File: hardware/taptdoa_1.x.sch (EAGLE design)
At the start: 67 parts, among them J1 105017-0001, U1 AP2112K-3.3TRG1, U2 STM32F103RBT6, Y1 8MHz

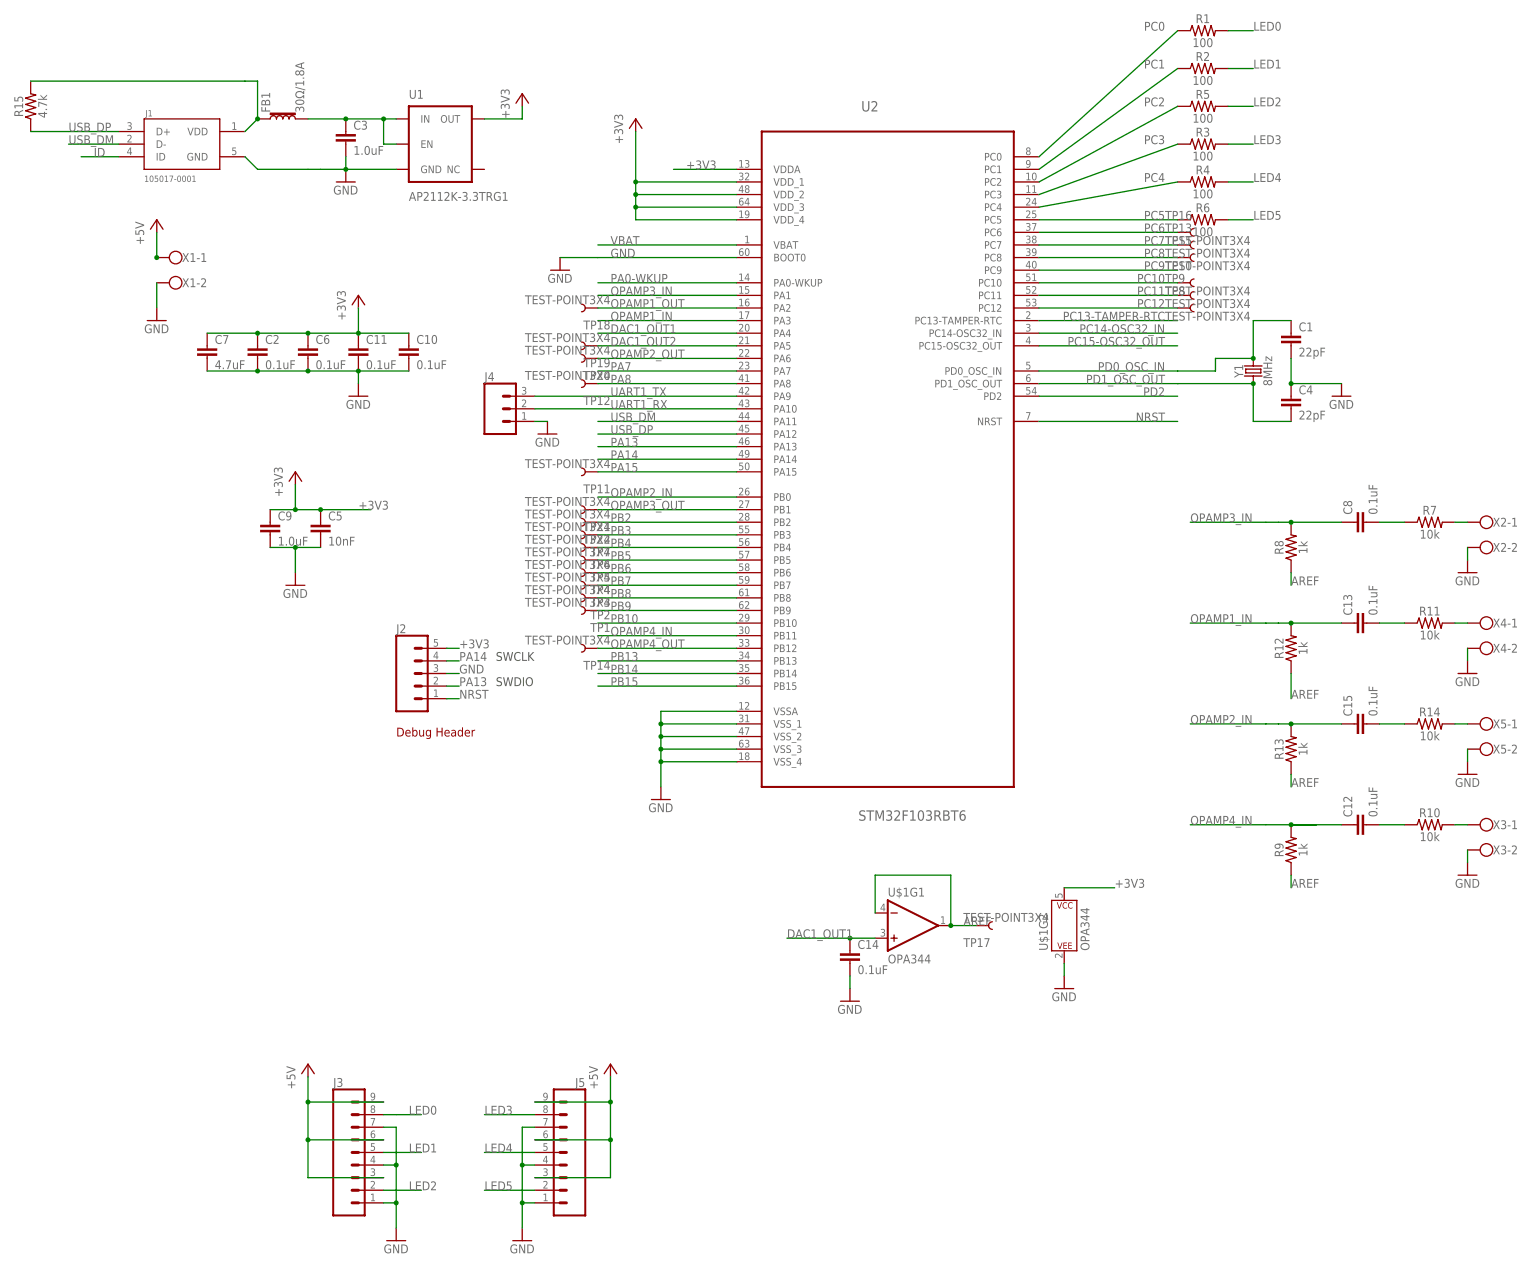
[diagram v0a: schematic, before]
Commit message: v1.2 of board
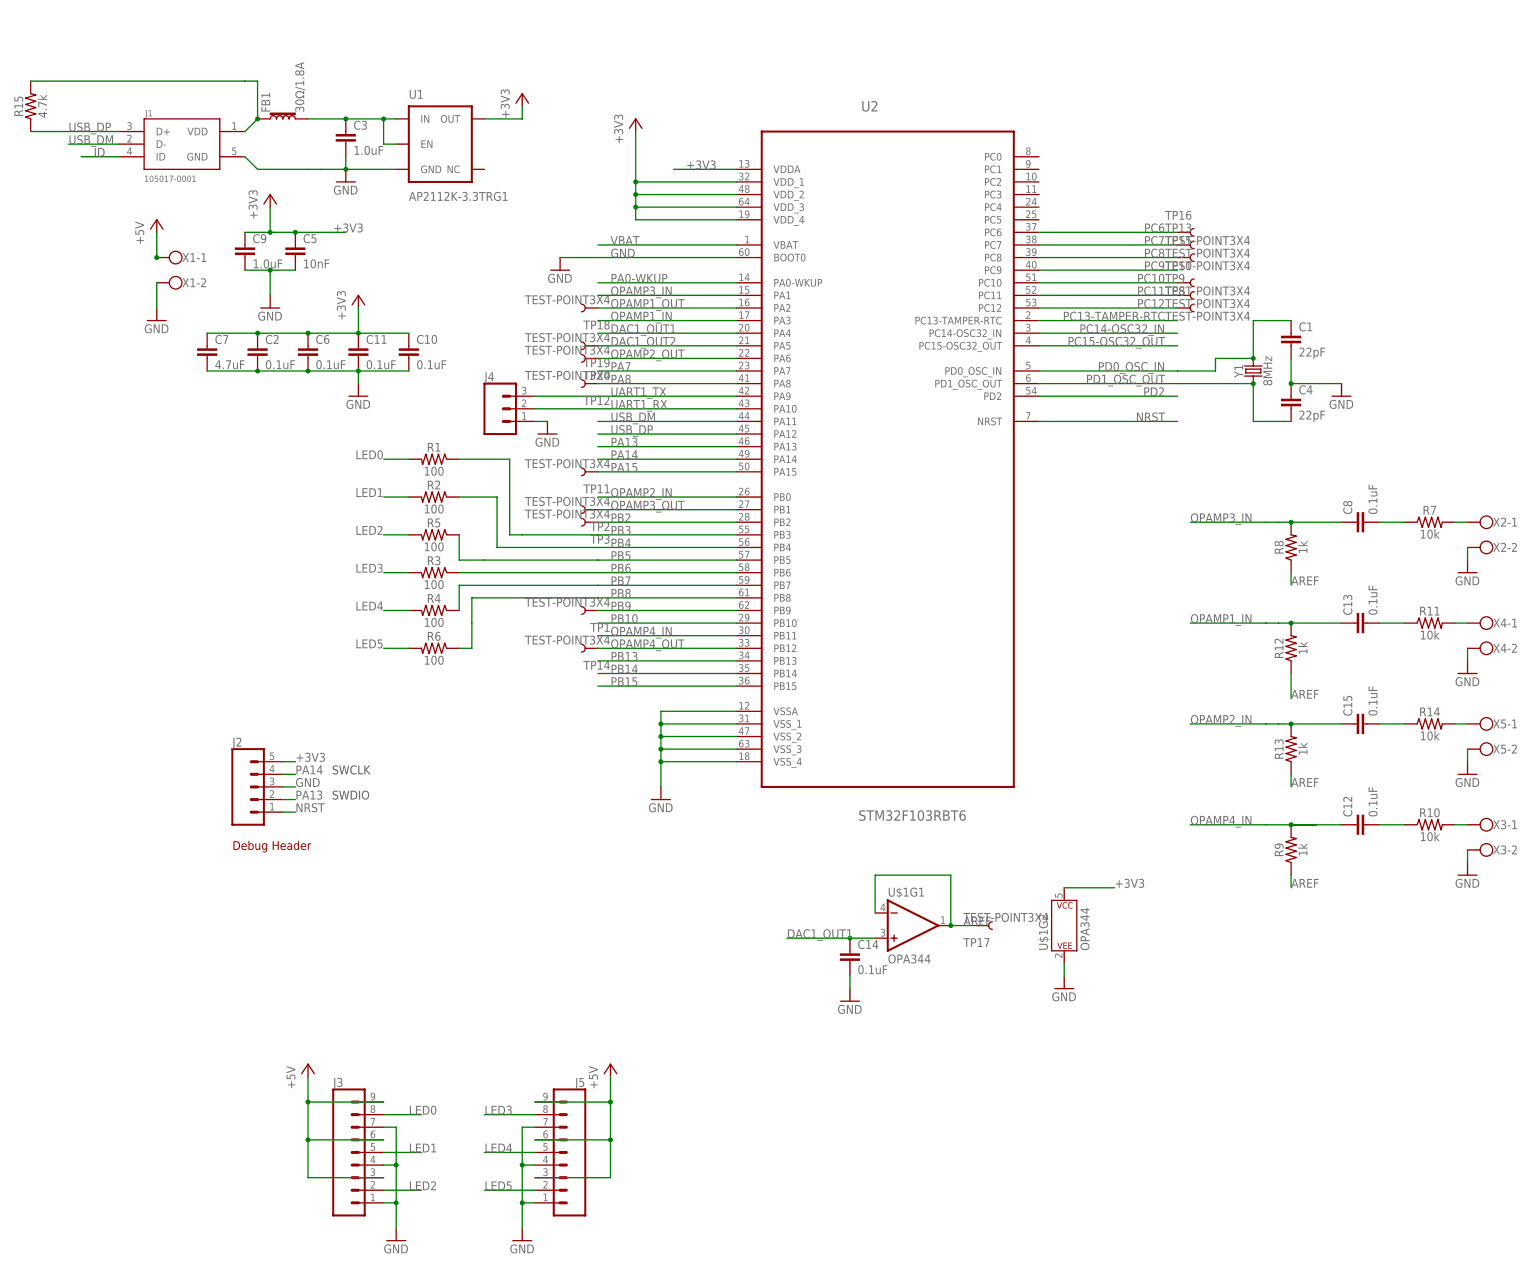
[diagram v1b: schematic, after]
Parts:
- removed TP21, TP22, TP4, TP5, TP6, TP7: TEST-POINT3X4, SparkFun-Connectors:TEST-POINT3X4
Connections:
- removed net PC0: R1.1, U2.PC0
- removed net PC1: R2.1, U2.PC1
- removed net PC2: R5.1, U2.PC2
- removed net PC3: R3.1, U2.PC3
- removed net PC4: R4.1, U2.PC4
- removed net PC5: R6.1, U2.PC5
- net OPAMP3_OUT: now also TP2.1; no longer TP21.1
- net PB2: now also TP3.1; no longer TP22.1
- net PB3: now also R1.1; no longer TP7.1
- net PB4: now also R2.1; no longer TP6.1
- net PB5: now also R5.1; no longer TP5.1
- net PB6: now also R3.1; no longer TP4.1
- net PB7: now also R4.1; no longer TP3.1
- net PB8: now also R6.1; no longer TP2.1
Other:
- moved on the sheet: C5, C9, J2, R1, R2, R3, R4, R5, R6, TP2, TP3
